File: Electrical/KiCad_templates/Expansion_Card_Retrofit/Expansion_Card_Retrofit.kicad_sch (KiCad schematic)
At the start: 15 parts, among them J1 Conn 10P, P1 USB_C_Plug_USB2.0, Q3 Q_Dual_NPN_NPN_C2E2C1E1B1B2, U1 AP7366EA-3.3, X1 ECS-2520MVLC-120-CM-TR

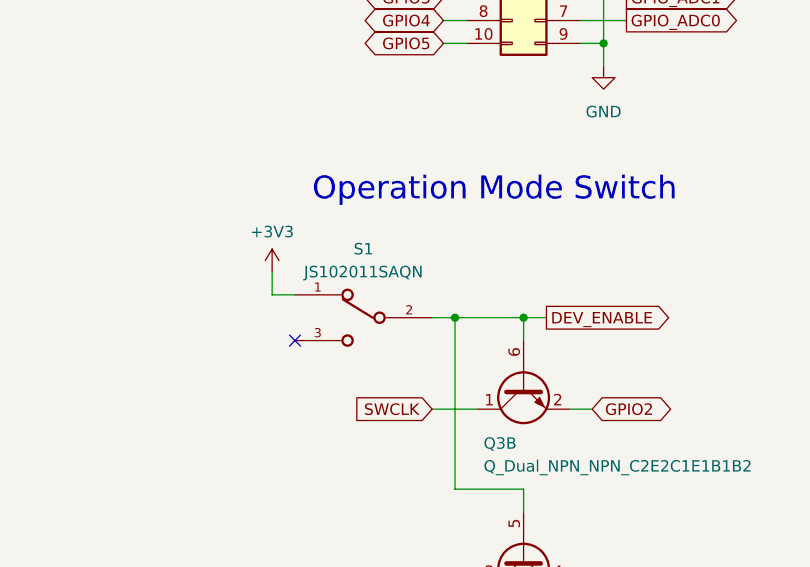
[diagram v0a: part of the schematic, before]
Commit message: Layout finished
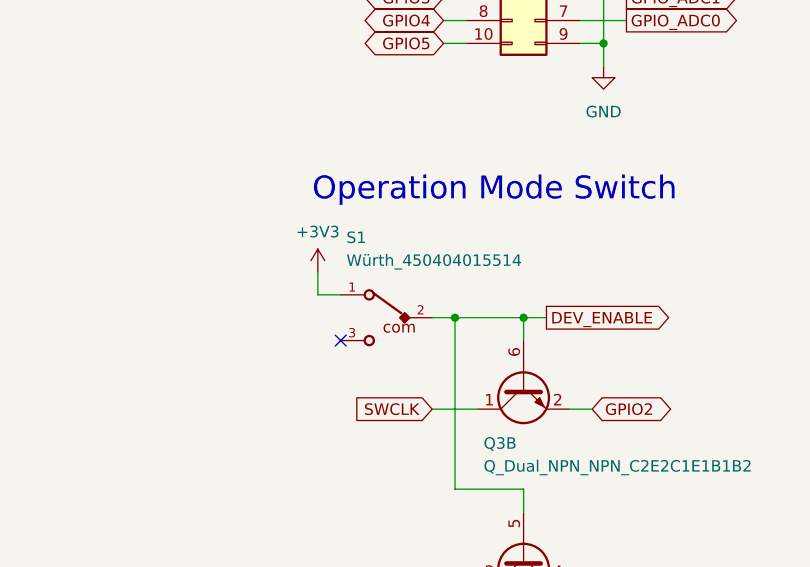
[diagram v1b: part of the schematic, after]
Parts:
- S1: value JS102011SAQN -> Würth_450404015514; footprint SnapEDA:SW_JS102011SAQN -> SnapEDA:450404015514; symbol SnapEDA:JS102011SAQN -> SnapEDA:450404015514; Check_prices https://www.snapeda.com/parts/JS102011SAQN/C%2526K/view-par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 -> https://www.snapeda.com/parts/450404015514/Wurth+Electronic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; DATASHEET-URL (none) -> https://www.we-online.com/catalog/datasheet/450404015514.pdf; IR (none) -> 300mA; MF C&K -> Wurth Electronics; MP JS102011SAQN -> 450404015514; PACKAGING (none) -> Tape and Reel; PART-NUMBER (none) -> 450404015514; Purchase-URL (none) -> https://www.snapeda.com/api/url_track_click_mouser/?unipart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; QTY (none) -> 150; SnapEDA_Link https://www.snapeda.com/parts/JS102011SAQN/C%2526K/view-par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 -> https://www.snapeda.com/parts/450404015514/Wurth+Electronic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; VR (none) -> 5V(DC)
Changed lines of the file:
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@@
   (no_connect (at 57.15 45.72))
   (no_connect (at 31.115 118.745))
-  (no_connect (at 217.805 101.6))
+  (no_connect (at 222.885 101.6))
   (wire (pts (xy 241.935 154.94) (xy 247.015 154.94))
     (stroke (width 0) (type default))
@@
     (stroke (width 0) (type default))
   )
-  (wire (pts (xy 215.265 96.52) (xy 217.805 96.52))
+  (wire (pts (xy 220.345 96.52) (xy 222.885 96.52))
     (stroke (width 0) (type default))
   )
@@
     (stroke (width 0) (type default))
   )
-  (wire (pts (xy 215.265 93.98) (xy 215.265 96.52))
+  (wire (pts (xy 220.345 93.98) (xy 220.345 96.52))
     (stroke (width 0) (type default))
   )
@@
     )
   )
-  (symbol (lib_id "power:+3V3") (at 215.265 93.98 0) (unit 1)
+  (symbol (lib_id "power:+3V3") (at 220.345 93.98 0) (unit 1)
     (in_bom yes) (on_board yes) (dnp no) (fields_autoplaced)
-    (property "Reference" "#PWR014" (at 215.265 97.79 0)
-      (effects (font (size 1.27 1.27)) hide)
-    )
-    (property "Value" "+3V3" (at 215.265 89.535 0)
-      (effects (font (size 1.27 1.27)))
-    )
-    (property "Footprint" "" (at 215.265 93.98 0)
-      (effects (font (size 1.27 1.27)) hide)
-    )
-    (property "Datasheet" "" (at 215.265 93.98 0)
+    (property "Reference" "#PWR014" (at 220.345 97.79 0)
+      (effects (font (size 1.27 1.27)) hide)
+    )
+    (property "Value" "+3V3" (at 220.345 89.535 0)
+      (effects (font (size 1.27 1.27)))
+    )
+    (property "Footprint" "" (at 220.345 93.98 0)
+      (effects (font (size 1.27 1.27)) hide)
+    )
+    (property "Datasheet" "" (at 220.345 93.98 0)
       (effects (font (size 1.27 1.27)) hide)
     )
@@
     )
   )
-  (symbol (lib_id "SnapEDA:JS102011SAQN") (at 225.425 99.06 0) (unit 1)
-    (in_bom yes) (on_board yes) (dnp no) (fields_autoplaced)
-    (property "Reference" "S1" (at 225.425 91.44 0)
-      (effects (font (size 1.27 1.27)))
-    )
-    (property "Value" "JS102011SAQN" (at 225.425 93.98 0)
-      (effects (font (size 1.27 1.27)))
-    )
-    (property "Footprint" "SnapEDA:SW_JS102011SAQN" (at 225.425 99.06 0)
-      (effects (font (size 1.27 1.27)) (justify bottom) hide)
-    )
-    (property "Datasheet" "" (at 225.425 99.06 0)
-      (effects (font (size 1.27 1.27)) hide)
-    )
-    (property "MF" "C&K" (at 225.425 99.06 0)
-      (effects (font (size 1.27 1.27)) (justify bottom) hide)
-    )
-    (property "Description" "\nSwitch, Slide, SPDT, ON-ON, 300mA, 6VDC, Surface Mount, R/A, Gull Wing | C&K JS102011SAQN\n" (at 225.425 99.06 0)
-      (effects (font (size 1.27 1.27)) (justify bottom) hide)
-    )
-    (property "Package" "None" (at 225.425 99.06 0)
-      (effects (font (size 1.27 1.27)) (justify bottom) hide)
-    )
-    (property "Price" "None" (at 225.425 99.06 0)
-      (effects (font (size 1.27 1.27)) (justify bottom) hide)
-    )
-    (property "Check_prices" "https://www.snapeda.com/parts/JS102011SAQN/C%2526K/view-part/?ref=eda" (at 225.425 99.06 0)
-      (effects (font (size 1.27 1.27)) (justify bottom) hide)
-    )
-    (property "SnapEDA_Link" "https://www.snapeda.com/parts/JS102011SAQN/C%2526K/view-part/?ref=snap" (at 225.425 99.06 0)
-      (effects (font (size 1.27 1.27)) (justify bottom) hide)
-    )
-    (property "MP" "JS102011SAQN" (at 225.425 99.06 0)
-      (effects (font (size 1.27 1.27)) (justify bottom) hide)
-    )
-    (property "Availability" "In Stock" (at 225.425 99.06 0)
-      (effects (font (size 1.27 1.27)) (justify bottom) hide)
-    )
-    (property "MANUFACTURER" "C&K" (at 225.425 99.06 0)
-      (effects (font (size 1.27 1.27)) (justify bottom) hide)
-    )
+  (symbol (lib_id "SnapEDA:450404015514") (at 227.965 99.06 0) (mirror y) (unit 1)
+    (in_bom yes) (on_board yes) (dnp no)
+    (property "Reference" "S1" (at 223.52 90.17 0)
+      (effects (font (size 1.27 1.27)) (justify right))
+    )
+    (property "Value" "Würth_450404015514" (at 223.52 92.71 0)
+      (effects (font (size 1.27 1.27)) (justify right))
+    )
+    (property "Footprint" "SnapEDA:450404015514" (at 227.965 99.06 0)
+      (effects (font (size 1.27 1.27)) (justify bottom) hide)
+    )
+    (property "Datasheet" "" (at 227.965 99.06 0)
+      (effects (font (size 1.27 1.27)) hide)
+    )
+    (property "MF" "Wurth Electronics" (at 227.965 99.06 0)
+      (effects (font (size 1.27 1.27)) (justify bottom) hide)
+    )
+    (property "Description" "\nMINI SLIDE SWITCH 6.7 X 2.7 MM.\n" (at 227.965 99.06 0)
+      (effects (font (size 1.27 1.27)) (justify bottom) hide)
+    )
+    (property "Package" "None" (at 227.965 99.06 0)
+      (effects (font (size 1.27 1.27)) (justify bottom) hide)
+    )
+    (property "Price" "None" (at 227.965 99.06 0)
+      (effects (font (size 1.27 1.27)) (justify bottom) hide)
+    )
+    (property "Check_prices" "https://www.snapeda.com/parts/450404015514/Wurth+Electronics+Inc./view-part/?ref=eda" (at 227.965 99.06 0)
+      (effects (font (size 1.27 1.27)) (justify bottom) hide)
+    )
+    (property "SnapEDA_Link" "https://www.snapeda.com/parts/450404015514/Wurth+Electronics+Inc./view-part/?ref=snap" (at 227.965 99.06 0)
+      (effects (font (size 1.27 1.27)) (justify bottom) hide)
+    )
+    (property "MP" "450404015514" (at 227.965 99.06 0)
+      (effects (font (size 1.27 1.27)) (justify bottom) hide)
+    )
+    (property "Availability" "In Stock" (at 227.965 99.06 0)
+      (effects (font (size 1.27 1.27)) (justify bottom) hide)
+    )
+    (property "MANUFACTURER" "C&K" (at 227.965 99.06 0)
+      (effects (font (size 1.27 1.27)) (justify bottom) hide)
+    )
+    (property "IR" "300mA" (at 227.965 99.06 0)
+      (effects (font (size 1.27 1.27)) (justify bottom) hide)
+    )
+    (property "QTY" "150" (at 227.965 99.06 0)
+      (effects (font (size 1.27 1.27)) (justify bottom) hide)
+    )
+    (property "PACKAGING" "Tape and Reel" (at 227.965 99.06 0)
+      (effects (font (size 1.27 1.27)) (justify bottom) hide)
+    )
+    (property "VR" "5V(DC)" (at 227.965 99.06 0)
+      (effects (font (size 1.27 1.27)) (justify bottom) hide)
+    )
+    (property "DATASHEET-URL" "https://www.we-online.com/catalog/datasheet/450404015514.pdf" (at 227.965 99.06 0)
+      (effects (font (size 1.27 1.27)) (justify bottom) hide)
+    )
+    (property "Purchase-URL" "https://www.snapeda.com/api/url_track_click_mouser/?unipart_id=3611018&manufacturer=Wurth Electronics&part_name=450404015514&search_term=450404015514" (at 227.965 99.06 0)
+      (effects (font (size 1.27 1.27)) (justify bottom) hide)
+    )
+    (property "PART-NUMBER" "450404015514" (at 227.965 99.06 0)
+      (effects (font (size 1.27 1.27)) (justify bottom) hide)
+    )
